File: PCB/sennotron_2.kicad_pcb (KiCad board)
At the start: 2 copper layers, 119 x 100 mm, 31 parts, among them J1 Barrel_Jack, J10 Conn_02x20_Odd_Even, J3 Conn_02x08_Odd_Even, J4 Conn_01x16_Female, J5 Screw_Terminal_01x02, J6 Screw_Terminal_01x16, J7 Conn_01x04_Male, J8 Conn_01x04_Male, J9 Conn_01x05_Female, U1 LM1117-3.3, U2 MCP3208, U3 S102S01, U4 4N28

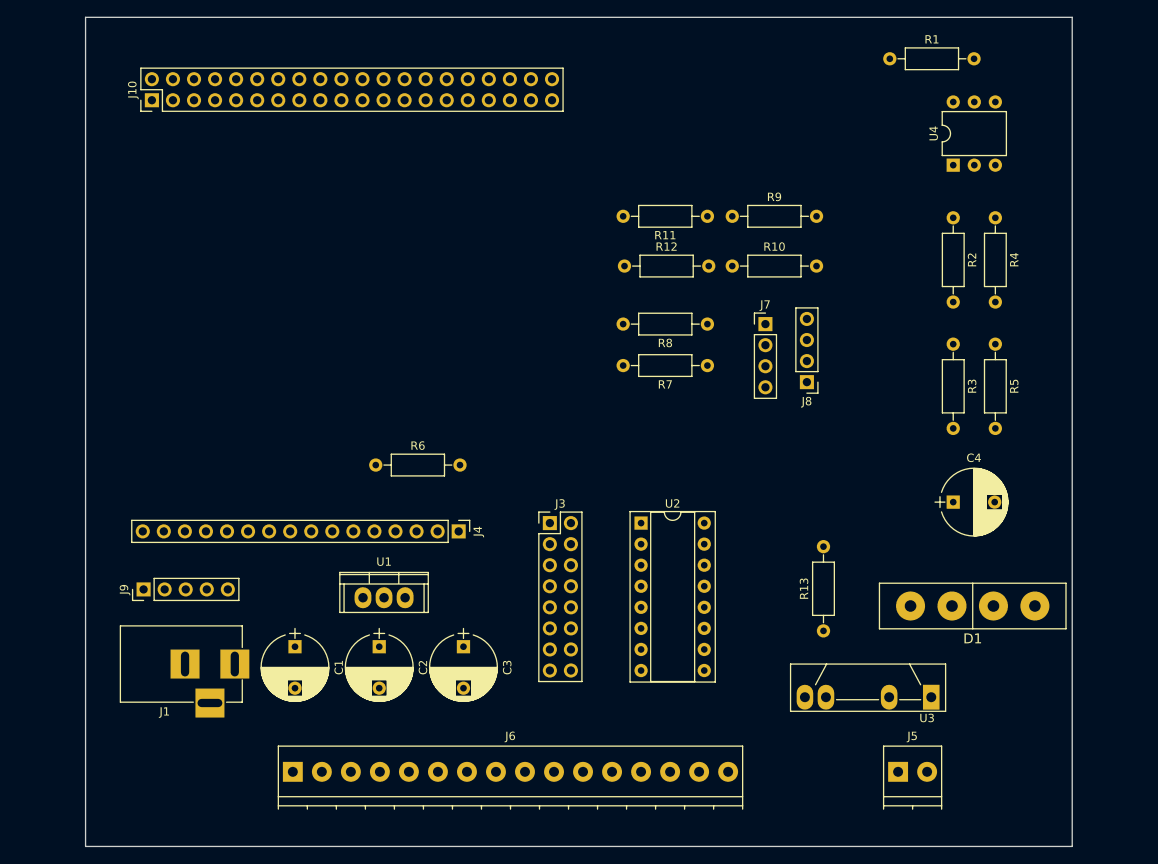
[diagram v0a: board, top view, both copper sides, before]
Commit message: pcb design almost done... waiting for a review!
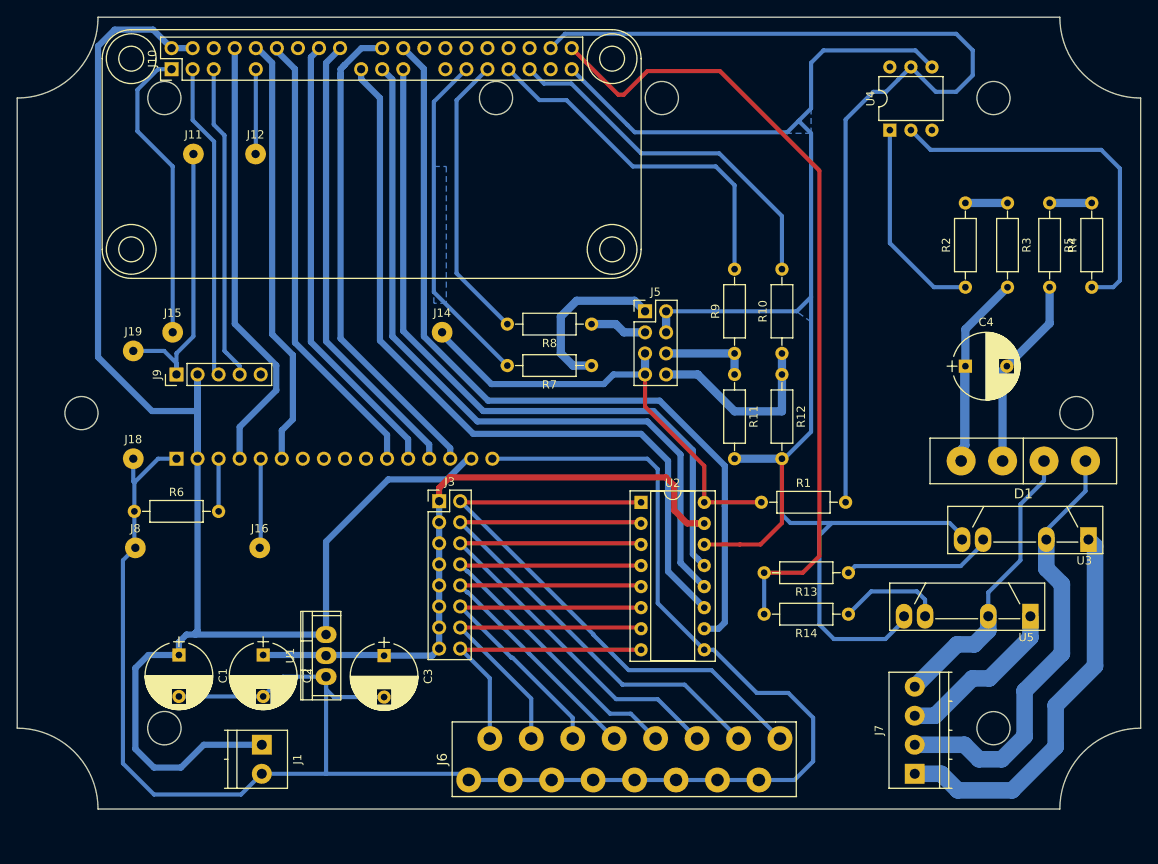
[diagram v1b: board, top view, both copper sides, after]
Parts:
- added J11: Conn_01x01, custom:Pad_2.5, F.Cu at (103.0, 65.5)
- added J12: Conn_01x01, custom:Pad_2.5, F.Cu at (110.5, 65.5)
- added J14: Conn_01x01, custom:Pad_2.5, F.Cu at (133.0, 87.0)
- added J15: Conn_01x01, custom:Pad_2.5, F.Cu at (100.5, 87.0)
- added J16: Conn_01x01, custom:Pad_2.5, F.Cu at (111.0, 113.0)
- added J18: Conn_01x01, custom:Pad_2.5, F.Cu at (95.8, 102.2)
- added J19: Conn_01x01, custom:Pad_2.5, F.Cu at (95.8, 89.2)
- added R14: R, Resistors_THT:R_Axial_DIN0207_L6.3mm_D2.5mm_P10.16mm_Horizontal, F.Cu at (182.0, 121.0)
- added U5: S102S01, Housings_SIP:SIP4_Sharp-SSR_Pitch7.62mm_Straight, F.Cu at (204.0, 121.2)
- J1: value Barrel_Jack -> Screw_Terminal_01x02; footprint Connectors:BARREL_JACK -> TerminalBlocks_Phoenix:TerminalBlock_Phoenix_PT-3.5mm_2pol
- J10: footprint Pin_Headers:Pin_Header_Straight_2x20_Pitch2.54mm -> custom:raspberry_pi_zero
- J4: moved to B.Cu
- J5: value Screw_Terminal_01x02 -> Conn_02x04_Odd_Even; footprint TerminalBlocks_Phoenix:TerminalBlock_Phoenix_PT-3.5mm_2pol -> Pin_Headers:Pin_Header_Straight_2x04_Pitch2.54mm
- J6: footprint TerminalBlocks_Phoenix:TerminalBlock_Phoenix_PT-3.5mm_16pol -> custom:springlock
- J7: value Conn_01x04_Male -> Screw_Terminal_01x04; footprint Pin_Headers:Pin_Header_Straight_1x04_Pitch2.54mm -> TerminalBlocks_Phoenix:TerminalBlock_Phoenix_PT-3.5mm_4pol
- J8: value Conn_01x04_Male -> Conn_01x01; footprint Pin_Headers:Pin_Header_Straight_1x04_Pitch2.54mm -> custom:Pad_2.5
- moved J8 83.4 mm to (96.0, 113.0), turned to 0 degrees
- moved J5 63.4 mm to (157.5, 84.5)
- moved J7 57.1 mm to (190.0, 140.2), turned to 90 degrees
- moved R1 55.7 mm to (171.5, 107.5)
- moved J6 38.7 mm to (153.7, 138.5)
- moved J4 35.1 mm to (101.0, 102.2)
- moved R6 29.6 mm to (95.9, 108.6)
- moved U3 26.8 mm to (211.0, 112.0)
- moved J9 26.2 mm to (101.0, 92.1)
- moved R12 23.1 mm to (174.0, 92.1), turned to 270 degrees
- moved R11 19.4 mm to (168.3, 92.1), turned to 270 degrees
- moved D1 18.5 mm to (203.1, 102.5)
- moved R5 18.2 mm to (206.3, 71.4)
- moved R3 18.2 mm to (201.2, 71.4)
- moved R9 16.5 mm to (168.3, 89.5), turned to 90 degrees
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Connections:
- D1 pad 3: /220L -> Net-(D1-Pad3)
- J10 pad 10: /lcd5 -> lcd_en
- J10 pad 12: /lcd4 -> lcd_d4
- J10 pad 14: (no net) -> Net-(J10-Pad14)
- J10 pad 16: /lcd3 -> lcd_d5
- J10 pad 18: /lcd2 -> lcd_d6
- J10 pad 22: /lcd1 -> lcd_d7
- J10 pad 26: (no net) -> Net-(J10-Pad26)
- J10 pad 27: (no net) -> Net-(J10-Pad27)
- J10 pad 28: (no net) -> Net-(J10-Pad28)
- J10 pad 30: GND -> Net-(J10-Pad30)
- J10 pad 32: (no net) -> Net-(J10-Pad32)
- J10 pad 34: GND -> Net-(J10-Pad34)
- J10 pad 36: (no net) -> Net-(J10-Pad36)
- J10 pad 37: (no net) -> Net-(J10-Pad37)
- J10 pad 38: heat_trig -> AC_sens
- J10 pad 40: AC_sens -> heat_trig
- J10 pad 6: GND -> Net-(J10-Pad6)
- J10 pad 8: /lcd6 -> lcd_rs
- J4 pad 10: (no net) -> Net-(J4-Pad10)
- J4 pad 11: /lcd3 -> lcd_d4
- J4 pad 12: /lcd4 -> lcd_d5
- J4 pad 13: /lcd5 -> lcd_d6
- J4 pad 14: /lcd6 -> lcd_d7
- J4 pad 4: /lcd1 -> lcd_rs
- J4 pad 6: /lcd2 -> lcd_en
- J4 pad 7: (no net) -> Net-(J4-Pad7)
- J4 pad 8: (no net) -> Net-(J4-Pad8)
- J4 pad 9: (no net) -> Net-(J4-Pad9)
- J5 pad 1: Net-(D1-Pad4) -> Net-(J5-Pad1)
- J5 pad 2: /220L -> GND
- J6 pad 1: Net-(J3-Pad2) -> GND
- J6 pad 10: GND -> Net-(J3-Pad8)
- J6 pad 11: Net-(J3-Pad12) -> GND
- J6 pad 12: GND -> Net-(J3-Pad6)
- J6 pad 13: Net-(J3-Pad14) -> GND
- J6 pad 14: GND -> Net-(J3-Pad4)
- J6 pad 15: Net-(J3-Pad16) -> GND
- J6 pad 16: GND -> Net-(J3-Pad2)
- J6 pad 2: GND -> Net-(J3-Pad16)
- J6 pad 3: Net-(J3-Pad4) -> GND
- J6 pad 4: GND -> Net-(J3-Pad14)
- J6 pad 5: Net-(J3-Pad6) -> GND
- J6 pad 6: GND -> Net-(J3-Pad12)
- J6 pad 7: Net-(J3-Pad8) -> GND
- J6 pad 8: GND -> Net-(J3-Pad10)
- J6 pad 9: Net-(J3-Pad10) -> GND
- J7 pad 2: GND -> Net-(D1-Pad4)
- J7 pad 3: GND -> Net-(J7-Pad3)
- J7 pad 4: Net-(J7-Pad4) -> Net-(D1-Pad3)
- J8 pad 1: Net-(J8-Pad1) -> GND
- J9 pad 5: (no net) -> Net-(J9-Pad5)
- R10 pad 1: Net-(J8-Pad1) -> Net-(J5-Pad8)
- R11 pad 1: Net-(J8-Pad4) -> Net-(J5-Pad6)
- R12 pad 1: GND -> Net-(J5-Pad8)
- R12 pad 2: Net-(J8-Pad1) -> GND
- R7 pad 1: Net-(J7-Pad4) -> Net-(J5-Pad1)
- R8 pad 1: Net-(J7-Pad1) -> Net-(J5-Pad3)
- R9 pad 1: Net-(J8-Pad4) -> Net-(J5-Pad6)
- U3 pad 1: Net-(D1-Pad4) -> Net-(J7-Pad1)
- U3 pad 2: /220L -> Net-(D1-Pad4)
- U4 pad 3: (no net) -> Net-(U4-Pad3)
- U4 pad 6: (no net) -> Net-(U4-Pad6)
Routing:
- net GND: track 0.00 -> 513.8 mm, vias 0 -> 4
- net +5V: track 0.00 -> 234.7 mm
- net +3.3VA: track 0.00 -> 134.6 mm
- net +3V3: track 0.00 -> 124.3 mm, vias 0 -> 3
- net AC_sens: track 0.00 -> 121.7 mm
- net spi_cs_0: track 0.00 -> 100.9 mm
- net heat_trig: track 0.00 -> 97.9 mm
- net spi_mosi: track 0.00 -> 93.9 mm
- net spi_miso: track 0.00 -> 90.5 mm
- net spi_clk: track 0.00 -> 86.9 mm
- net Net-(J3-Pad2): track 0.00 -> 72.5 mm, vias 0 -> 2
- net Net-(J3-Pad4): track 0.00 -> 66.5 mm
- net Net-(J3-Pad6): track 0.00 -> 60.2 mm
- net lcd_d7: track 0.00 -> 59.4 mm
- net lcd_d6: track 0.00 -> 55.4 mm
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- added copper zone on B.Cu, net GND
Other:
- board size 119 x 100 mm -> 135.5 x 95.5 mm
- copper layers 2 -> 4
- net class 5v added: clearance 0.2, trace_width 0.75, via_dia 0.6, via_drill 0.4
- net class AC added: clearance 0.5, trace_width 2, via_dia 0.6, via_drill 0.4
- net class Default: trace_width 0.25 -> 0.5
- net class lcd added: clearance 0.2, trace_width 0.75, via_dia 0.6, via_drill 0.4
- rule trace_min: 0.2 -> 0.5
